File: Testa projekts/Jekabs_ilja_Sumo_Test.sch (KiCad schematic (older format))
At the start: 1 part

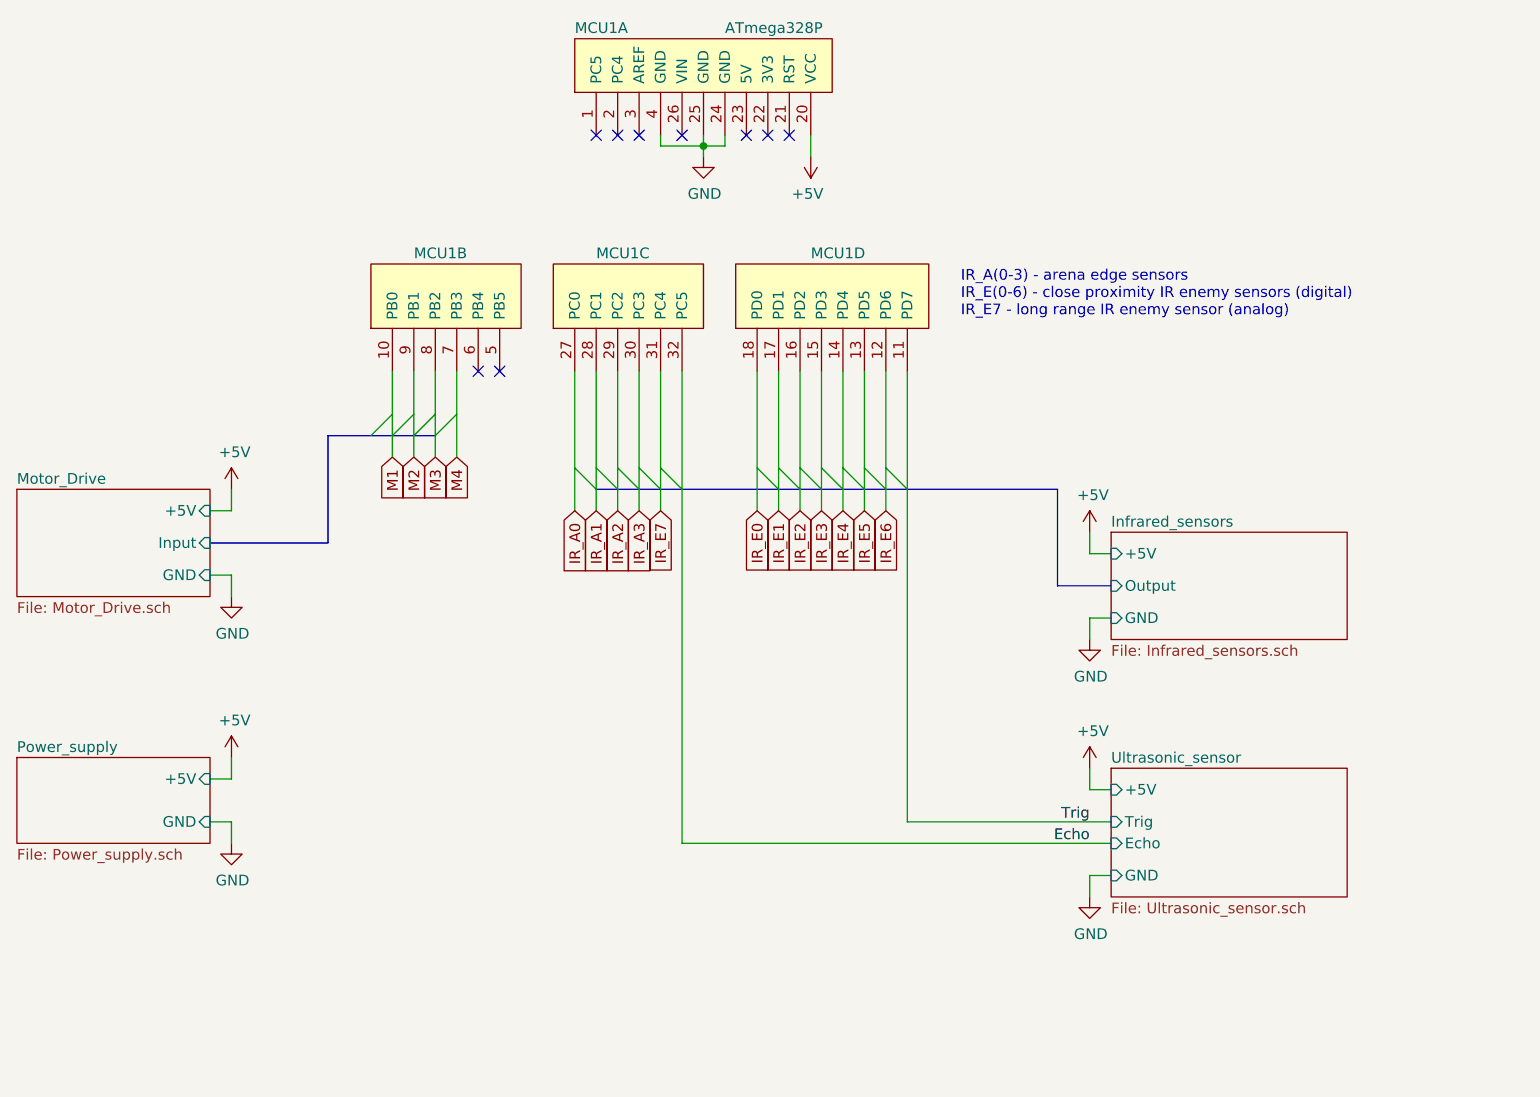
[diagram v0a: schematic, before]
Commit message: Testa principiālās shēmas pdf sagatave
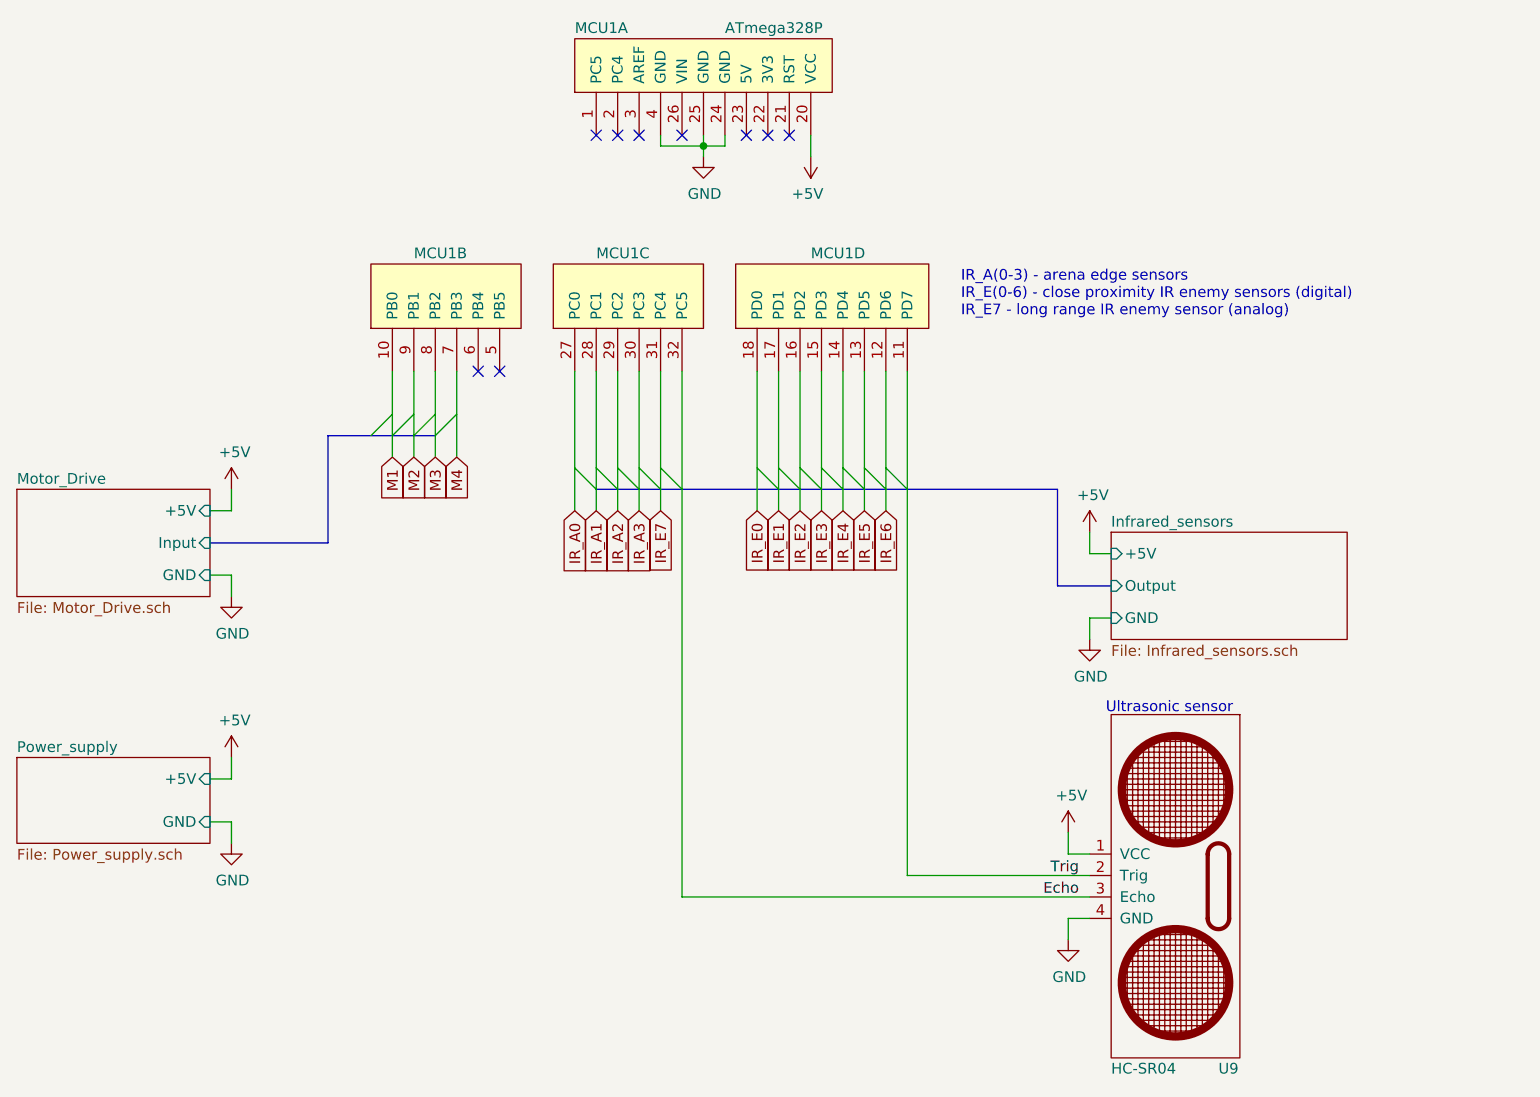
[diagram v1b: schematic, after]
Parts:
- added U9: HC-SR04, Socket_Strips:Socket_Strip_Straight_1x04_Pitch2.54mm, symbol Custom_draws:HC-SR04
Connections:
- net +5V: now also U9.1 (VCC)
- net Echo: now also U9.3 (Echo)
- net GND: now also U9.4 (GND)
- net Trig: now also U9.2 (Trig)
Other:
- note added: "Ultrasonic sensor"
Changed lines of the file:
@@
 EESchema Schematic File Version 4
-LIBS:Sumo bot-cache
+LIBS:Jekabs_Ilja_Sumo_Test-cache
 EELAYER 26 0
 EELAYER END
 $Descr A4 11693 8268
 encoding utf-8
-Sheet 1 5
+Sheet 1 4
 Title ""
 Date ""
@@
 F4 "GND" I R 3150 3600 50
 $EndSheet
-$Sheet
-S 7350 4500 1100 600
-U 605AB373
-F0 "Ultrasonic_sensor" 50
-F1 "Ultrasonic_sensor.sch" 50
-F2 "+5V" I L 7350 4600 50
-F3 "GND" I L 7350 5000 50
-F4 "Trig" I L 7350 4750 50
-F5 "Echo" I L 7350 4850 50
-$EndSheet
-$Comp
-L power:GND #PWR06
-U 1 1 605AC66A
-P 7250 5100
-F 0 "#PWR06" H 7250 4850 50  0001 C CNN
-F 1 "GND" H 7255 4927 50  0000 C CNN
-F 2 "" H 7250 5100 50  0001 C CNN
-F 3 "" H 7250 5100 50  0001 C CNN
-	1    7250 5100
-	1    0    0    -1
-$EndComp
-$Comp
-L power:+5V #PWR05
-U 1 1 605AC67D
-P 7250 4500
-F 0 "#PWR05" H 7250 4350 50  0001 C CNN
-F 1 "+5V" H 7265 4673 50  0000 C CNN
-F 2 "" H 7250 4500 50  0001 C CNN
-F 3 "" H 7250 4500 50  0001 C CNN
-	1    7250 4500
-	1    0    0    -1
-$EndComp
-Wire Wire Line
-	7350 4600 7250 4600
-Wire Wire Line
-	7250 4600 7250 4500
-Wire Wire Line
-	7350 5000 7250 5000
-Wire Wire Line
-	7250 5000 7250 5100
 Entry Wire Line
 	4850 3100 4950 3200
@@
 Wire Bus Line
 	7100 3200 7100 3650
-Wire Wire Line
-	6400 4750 7350 4750
-Text Label 7250 4750 2    50   ~ 0
+Text Label 7200 5000 2    50   ~ 0
 Trig
-Text Label 7250 4850 2    50   ~ 0
+Text Label 7200 5100 2    50   ~ 0
 Echo
 Wire Bus Line
@@
 	0    -1   -1   0
 $EndComp
-Wire Wire Line
-	5350 4850 7350 4850
 Entry Wire Line
 	5250 3100 5350 3200
@@
 Wire Wire Line
 	4300 2650 4300 3050
-Wire Wire Line
-	6400 2650 6400 4750
-Wire Wire Line
-	5350 2650 5350 4850
+Wire Bus Line
+	4950 3200 7100 3200
+$Comp
+L Custom_draws:HC-SR04 U?
+U 1 1 605CB393
+P 7650 5050
+AR Path="/605AB373/605CB393" Ref="U?"  Part="1"
+AR Path="/605CB393" Ref="U9"  Part="1"
+F 0 "U9" V 8500 5250 50  0000 L CNN
+F 1 "HC-SR04" V 8500 4750 50  0000 L CNN
+F 2 "Socket_Strips:Socket_Strip_Straight_1x04_Pitch2.54mm" H 7600 5050 50  0001 C CNN
+F 3 "" H 7600 5050 50  0001 C CNN
+	1    7650 5050
+	0    1    1    0
+$EndComp
+Wire Wire Line
+	6400 2650 6400 5000
+Wire Wire Line
+	5350 2650 5350 5100
+Wire Wire Line
+	5350 5100 7250 5100
+Wire Wire Line
+	6400 5000 7250 5000
+$Comp
+L power:GND #PWR0109
+U 1 1 605ED709
+P 7150 5300
+F 0 "#PWR0109" H 7150 5050 50  0001 C CNN
+F 1 "GND" H 7155 5127 50  0000 C CNN
+F 2 "" H 7150 5300 50  0001 C CNN
+F 3 "" H 7150 5300 50  0001 C CNN
+	1    7150 5300
+	1    0    0    -1
+$EndComp
+Wire Wire Line
+	7250 5200 7150 5200
+Wire Wire Line
+	7150 5200 7150 5300
+$Comp
+L power:+5V #PWR0110
+U 1 1 605EE87B
+P 7150 4800
+F 0 "#PWR0110" H 7150 4650 50  0001 C CNN
+F 1 "+5V" H 7165 4973 50  0000 C CNN
+F 2 "" H 7150 4800 50  0001 C CNN
+F 3 "" H 7150 4800 50  0001 C CNN
+	1    7150 4800
+	1    0    0    -1
+$EndComp
+Wire Wire Line
+	7250 4900 7150 4900
+Wire Wire Line
+	7150 4800 7150 4900
+Wire Wire Line
+	6300 2650 6300 3300
+Wire Wire Line
+	6200 2650 6200 3300
+Wire Wire Line
+	6000 2650 6000 3300
+Wire Wire Line
+	6100 2650 6100 3300
+Wire Wire Line
+	5900 2650 5900 3300
+Wire Wire Line
+	5800 2650 5800 3300
+Wire Wire Line
+	5150 2650 5150 3300
+Wire Wire Line
+	5250 2650 5250 3300
+Wire Wire Line
+	5050 2650 5050 3300
+Wire Wire Line
+	4950 2650 4950 3300
+Wire Wire Line
+	4200 2650 4200 3050
+Wire Wire Line
+	4100 2650 4100 3050
+Wire Wire Line
+	4000 2650 4000 3050
+Wire Wire Line
+	4850 2650 4850 3300
 Wire Wire Line
 	5700 2650 5700 3300
-Wire Wire Line
-	4850 2650 4850 3300
-Wire Wire Line
-	4000 2650 4000 3050
-Wire Wire Line
-	4100 2650 4100 3050
-Wire Wire Line
-	4200 2650 4200 3050
-Wire Wire Line
-	4950 2650 4950 3300
-Wire Wire Line
-	5050 2650 5050 3300
-Wire Wire Line
-	5250 2650 5250 3300
-Wire Wire Line
-	5150 2650 5150 3300
-Wire Wire Line
-	5800 2650 5800 3300
-Wire Wire Line
-	5900 2650 5900 3300
-Wire Wire Line
-	6100 2650 6100 3300
-Wire Wire Line
-	6000 2650 6000 3300
-Wire Wire Line
-	6200 2650 6200 3300
-Wire Wire Line
-	6300 2650 6300 3300
 Wire Bus Line
 	3700 2950 4200 2950
-Wire Bus Line
-	4950 3200 7100 3200
+Text Notes 7325 4250 0    50   ~ 0
+Ultrasonic sensor
 $EndSCHEMATC
